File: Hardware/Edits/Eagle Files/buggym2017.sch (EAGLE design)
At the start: 6 parts, among them IC1 4001N, IC2 4075N, IC3 BCC, IC4 L293E

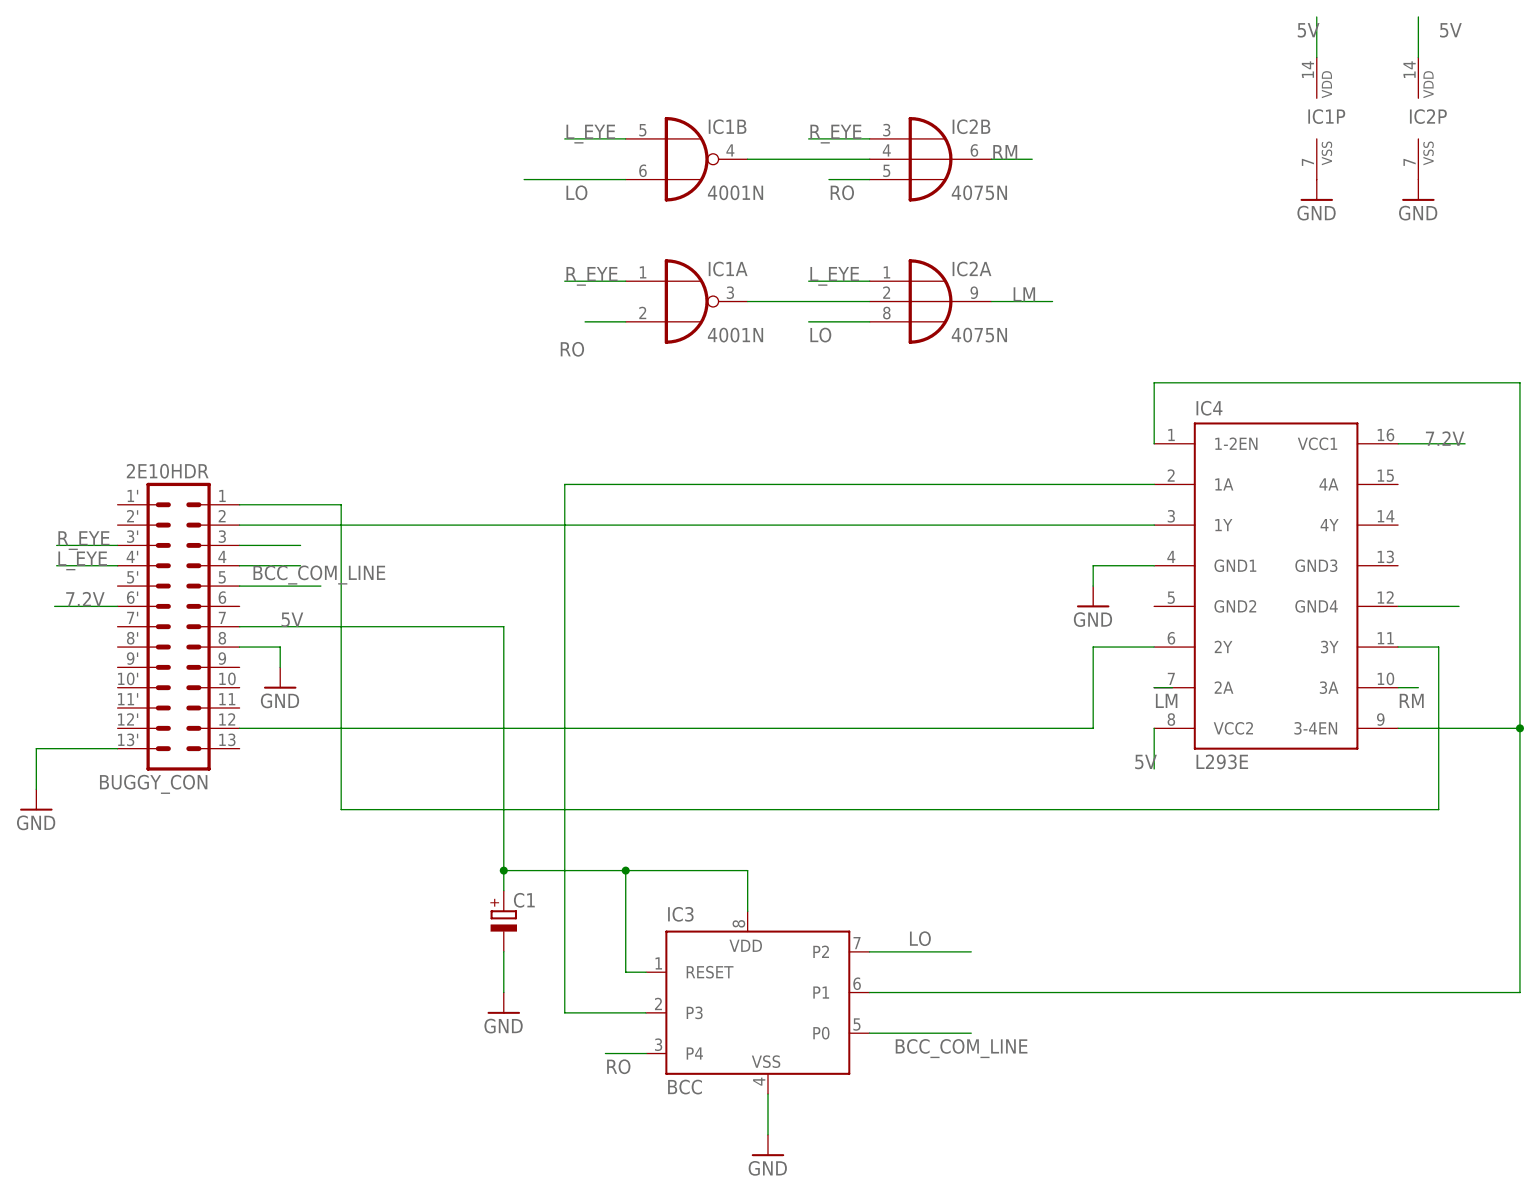
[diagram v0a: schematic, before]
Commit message: Work Done in Week 3  HardwareLab
Work done in Multisim and Eagle
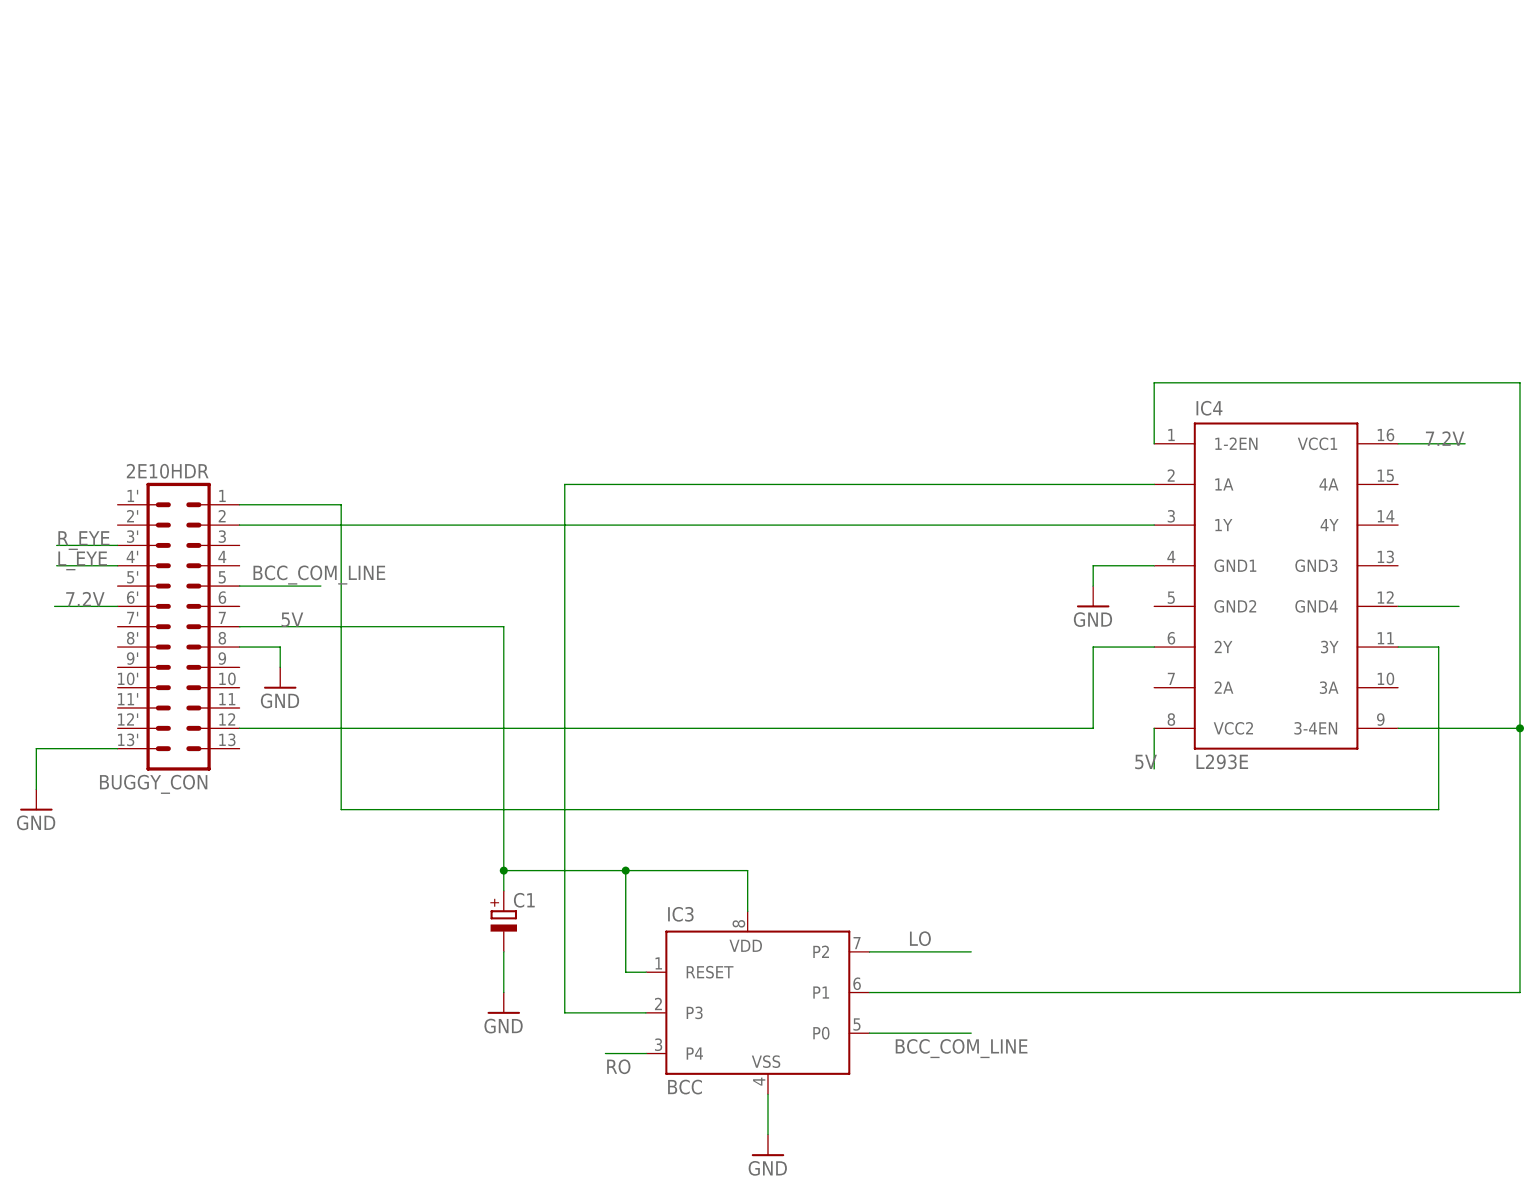
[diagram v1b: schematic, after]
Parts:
- removed IC1: 4001N, 40xx:4001N
- removed IC2: 4075N, 40xx:4075N
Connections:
- removed net LM: IC2A.O
- removed net N$1: IC1A.O, IC2A.I1
- removed net N$4: IC1B.O, IC2B.I1
- removed net RM: IC2B.O
- net GND: no longer IC1P.VSS, IC2P.VSS
- net L_EYE: no longer BUGGY_CON.4
- net R_EYE: no longer BUGGY_CON.3
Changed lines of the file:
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@@
 <?xml version="1.0" encoding="utf-8"?>
 <!DOCTYPE eagle SYSTEM "eagle.dtd">
-<eagle version="7.7.0">
+<eagle version="7.3.0">
 <drawing>
 <settings>
@@
 <part name="GND1" library="supply1" deviceset="GND" device=""/>
 <part name="GND3" library="supply1" deviceset="GND" device=""/>
-<part name="IC1" library="40xx" deviceset="4001" device="N"/>
-<part name="IC2" library="40xx" deviceset="4075" device="N"/>
-<part name="GND4" library="supply1" deviceset="GND" device=""/>
-<part name="GND5" library="supply1" deviceset="GND" device=""/>
 </parts>
 <sheets>
@@
 <instance part="GND1" gate="1" x="-35.56" y="15.24"/>
 <instance part="GND3" gate="1" x="-66.04" y="0"/>
-<instance part="IC1" gate="A" x="15.24" y="63.5"/>
-<instance part="IC2" gate="A" x="45.72" y="63.5"/>
-<instance part="IC2" gate="B" x="45.72" y="81.28"/>
-<instance part="IC1" gate="B" x="15.24" y="81.28"/>
-<instance part="IC1" gate="P" x="93.98" y="86.36"/>
-<instance part="IC2" gate="P" x="106.68" y="86.36"/>
-<instance part="GND4" gate="1" x="93.98" y="76.2"/>
-<instance part="GND5" gate="1" x="106.68" y="76.2"/>
 </instances>
 <busses>
@@
 <wire x1="38.1" y1="-17.78" x2="50.8" y2="-17.78" width="0.1524" layer="91"/>
 <label x="42.926" y="-17.018" size="1.778" layer="95"/>
-</segment>
-<segment>
-<wire x1="30.48" y1="60.96" x2="38.1" y2="60.96" width="0.1524" layer="91"/>
-<label x="30.48" y="58.42" size="1.778" layer="95"/>
-</segment>
-<segment>
-<wire x1="-5.08" y1="78.74" x2="7.62" y2="78.74" width="0.1524" layer="91"/>
-<label x="0" y="76.2" size="1.778" layer="95"/>
 </segment>
 </net>
@@
 <wire x1="-7.62" y1="22.86" x2="-40.64" y2="22.86" width="0.1524" layer="91"/>
 </segment>
-<segment>
-<wire x1="93.98" y1="99.06" x2="93.98" y2="93.98" width="0.1524" layer="91"/>
-<label x="91.44" y="96.52" size="1.778" layer="95"/>
-</segment>
-<segment>
-<wire x1="106.68" y1="93.98" x2="106.68" y2="99.06" width="0.1524" layer="91"/>
-<label x="109.22" y="96.52" size="1.778" layer="95"/>
-</segment>
 </net>
 <net name="GND" class="0">
@@
 <pinref part="BUGGY_CON" gate="G$1" pin="13'"/>
 <wire x1="-66.04" y1="7.62" x2="-55.88" y2="7.62" width="0.1524" layer="91"/>
-</segment>
-<segment>
-<pinref part="IC1" gate="P" pin="VSS"/>
-<pinref part="GND4" gate="1" pin="GND"/>
-</segment>
-<segment>
-<pinref part="IC2" gate="P" pin="VSS"/>
-<pinref part="GND5" gate="1" pin="GND"/>
 </segment>
 </net>
@@
 <label x="5.08" y="-33.02" size="1.778" layer="95"/>
 </segment>
-<segment>
-<wire x1="2.54" y1="60.96" x2="7.62" y2="60.96" width="0.1524" layer="91"/>
-<label x="2.54" y="58.42" size="1.778" layer="95" rot="R180"/>
-</segment>
-<segment>
-<wire x1="33.02" y1="78.74" x2="38.1" y2="78.74" width="0.1524" layer="91"/>
-<label x="33.02" y="76.2" size="1.778" layer="95"/>
-</segment>
 </net>
 <net name="R_EYE" class="0">
@@
 <label x="-63.5" y="33.02" size="1.778" layer="95"/>
 </segment>
-<segment>
-<wire x1="7.62" y1="66.04" x2="0" y2="66.04" width="0.1524" layer="91"/>
-<label x="0" y="66.04" size="1.778" layer="95"/>
-</segment>
-<segment>
-<pinref part="BUGGY_CON" gate="G$1" pin="3"/>
-<wire x1="-33.02" y1="33.02" x2="-40.64" y2="33.02" width="0.1524" layer="91"/>
-</segment>
-<segment>
-<wire x1="38.1" y1="83.82" x2="30.48" y2="83.82" width="0.1524" layer="91"/>
-<label x="30.48" y="83.82" size="1.778" layer="95"/>
-</segment>
 </net>
 <net name="L_EYE" class="0">
@@
 <wire x1="-55.88" y1="30.48" x2="-63.5" y2="30.48" width="0.1524" layer="91"/>
 <label x="-63.5" y="30.48" size="1.778" layer="95"/>
-</segment>
-<segment>
-<wire x1="30.48" y1="66.04" x2="38.1" y2="66.04" width="0.1524" layer="91"/>
-<label x="30.48" y="66.04" size="1.778" layer="95"/>
-</segment>
-<segment>
-<pinref part="BUGGY_CON" gate="G$1" pin="4"/>
-<wire x1="-40.64" y1="30.48" x2="-33.02" y2="30.48" width="0.1524" layer="91"/>
-</segment>
-<segment>
-<wire x1="0" y1="83.82" x2="7.62" y2="83.82" width="0.1524" layer="91"/>
-<label x="0" y="83.82" size="1.778" layer="95"/>
 </segment>
 </net>
@@
 </segment>
 </net>
-<net name="N$1" class="0">
-<segment>
-<pinref part="IC1" gate="A" pin="O"/>
-<pinref part="IC2" gate="A" pin="I1"/>
-<wire x1="22.86" y1="63.5" x2="38.1" y2="63.5" width="0.1524" layer="91"/>
-</segment>
-</net>
-<net name="LM" class="0">
-<segment>
-<pinref part="IC2" gate="A" pin="O"/>
-<wire x1="53.34" y1="63.5" x2="60.96" y2="63.5" width="0.1524" layer="91"/>
-<label x="55.88" y="63.5" size="1.778" layer="95"/>
-</segment>
-<segment>
-<wire x1="75.946" y1="15.24" x2="73.66" y2="15.24" width="0.1524" layer="91"/>
-<label x="73.66" y="12.7" size="1.778" layer="95"/>
-</segment>
-</net>
-<net name="RM" class="0">
-<segment>
-<pinref part="IC2" gate="B" pin="O"/>
-<wire x1="53.34" y1="81.28" x2="58.42" y2="81.28" width="0.1524" layer="91"/>
-<label x="53.34" y="81.28" size="1.778" layer="95"/>
-</segment>
-<segment>
-<wire x1="104.14" y1="15.24" x2="106.68" y2="15.24" width="0.1524" layer="91"/>
-<label x="104.14" y="12.7" size="1.778" layer="95"/>
-</segment>
-</net>
-<net name="N$4" class="0">
-<segment>
-<pinref part="IC1" gate="B" pin="O"/>
-<pinref part="IC2" gate="B" pin="I1"/>
-<wire x1="22.86" y1="81.28" x2="38.1" y2="81.28" width="0.1524" layer="91"/>
-</segment>
-</net>

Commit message: Tidy
Tidied up filesystem from HW Lab Week 3
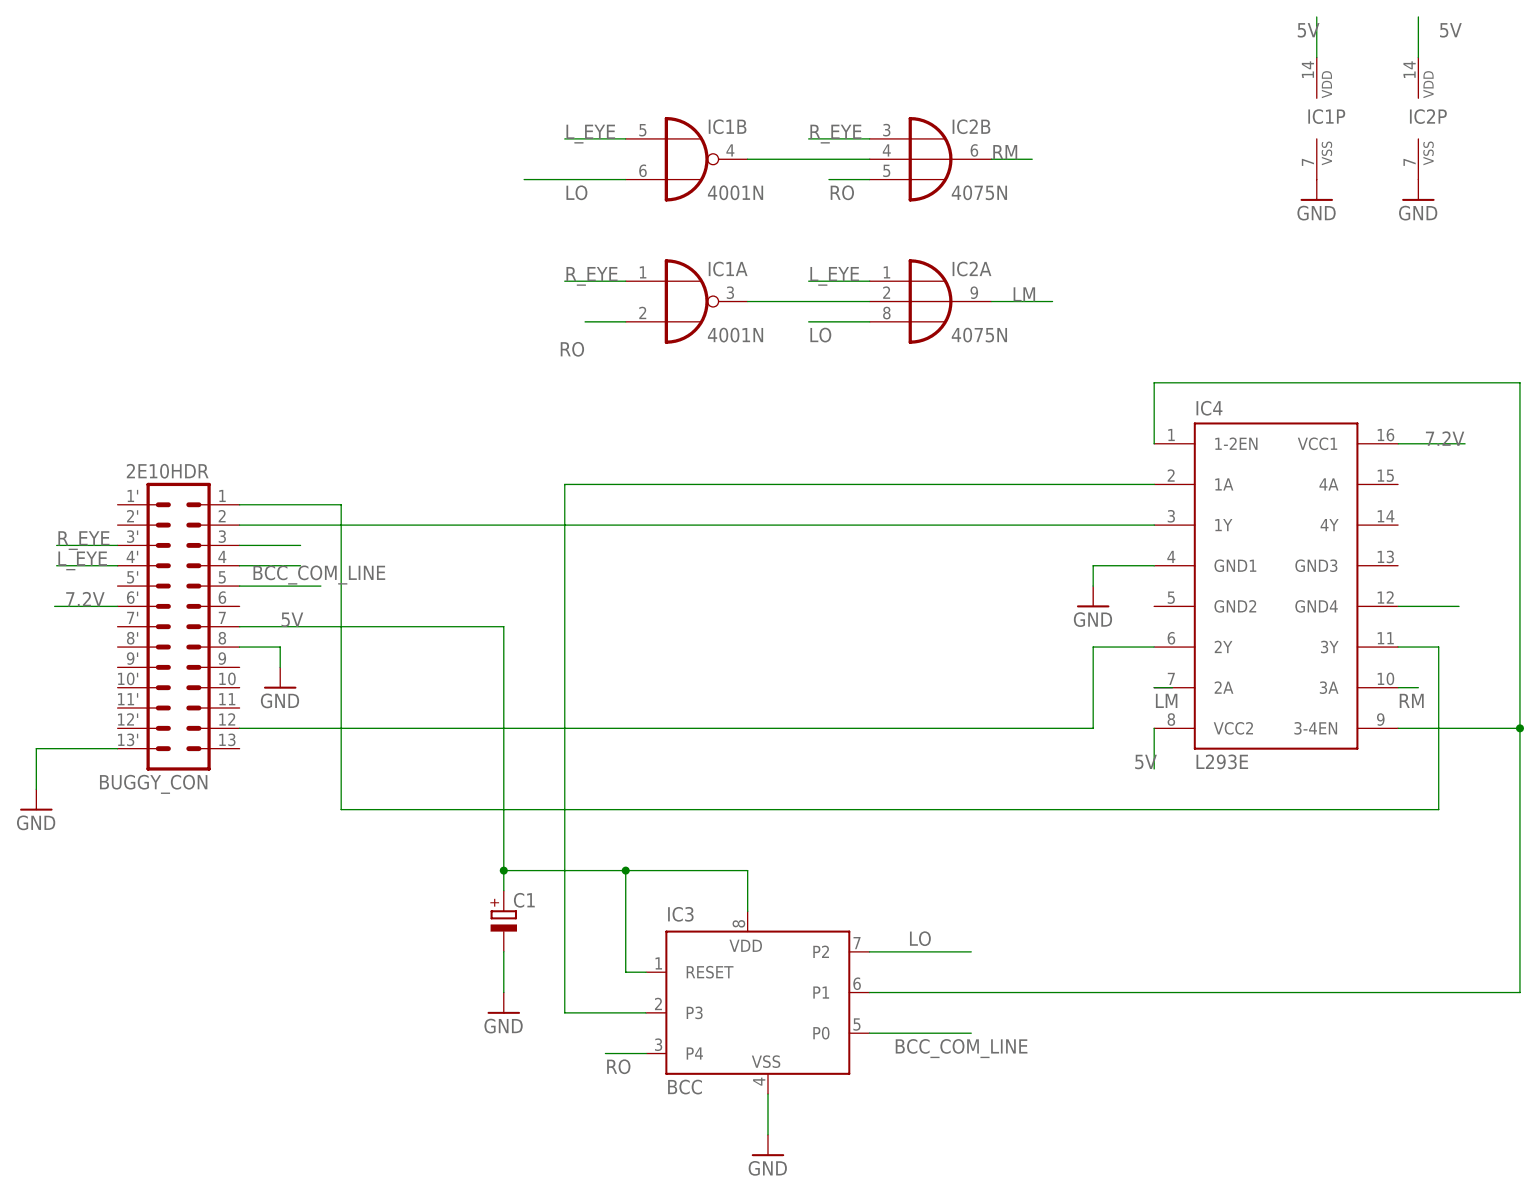
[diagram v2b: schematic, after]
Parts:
- added IC1: 4001N, 40xx:4001N
- added IC2: 4075N, 40xx:4075N
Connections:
- new net LM: IC2A.O
- new net N$1: IC1A.O, IC2A.I1
- new net N$4: IC1B.O, IC2B.I1
- new net RM: IC2B.O
- net GND: now also IC1P.VSS, IC2P.VSS
- net L_EYE: now also BUGGY_CON.4
- net R_EYE: now also BUGGY_CON.3
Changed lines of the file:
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@@
 <?xml version="1.0" encoding="utf-8"?>
 <!DOCTYPE eagle SYSTEM "eagle.dtd">
-<eagle version="7.3.0">
+<eagle version="7.7.0">
 <drawing>
 <settings>
@@
 <part name="GND1" library="supply1" deviceset="GND" device=""/>
 <part name="GND3" library="supply1" deviceset="GND" device=""/>
+<part name="IC1" library="40xx" deviceset="4001" device="N"/>
+<part name="IC2" library="40xx" deviceset="4075" device="N"/>
+<part name="GND4" library="supply1" deviceset="GND" device=""/>
+<part name="GND5" library="supply1" deviceset="GND" device=""/>
 </parts>
 <sheets>
@@
 <instance part="GND1" gate="1" x="-35.56" y="15.24"/>
 <instance part="GND3" gate="1" x="-66.04" y="0"/>
+<instance part="IC1" gate="A" x="15.24" y="63.5"/>
+<instance part="IC2" gate="A" x="45.72" y="63.5"/>
+<instance part="IC2" gate="B" x="45.72" y="81.28"/>
+<instance part="IC1" gate="B" x="15.24" y="81.28"/>
+<instance part="IC1" gate="P" x="93.98" y="86.36"/>
+<instance part="IC2" gate="P" x="106.68" y="86.36"/>
+<instance part="GND4" gate="1" x="93.98" y="76.2"/>
+<instance part="GND5" gate="1" x="106.68" y="76.2"/>
 </instances>
 <busses>
@@
 <wire x1="38.1" y1="-17.78" x2="50.8" y2="-17.78" width="0.1524" layer="91"/>
 <label x="42.926" y="-17.018" size="1.778" layer="95"/>
+</segment>
+<segment>
+<wire x1="30.48" y1="60.96" x2="38.1" y2="60.96" width="0.1524" layer="91"/>
+<label x="30.48" y="58.42" size="1.778" layer="95"/>
+</segment>
+<segment>
+<wire x1="-5.08" y1="78.74" x2="7.62" y2="78.74" width="0.1524" layer="91"/>
+<label x="0" y="76.2" size="1.778" layer="95"/>
 </segment>
 </net>
@@
 <wire x1="-7.62" y1="22.86" x2="-40.64" y2="22.86" width="0.1524" layer="91"/>
 </segment>
+<segment>
+<wire x1="93.98" y1="99.06" x2="93.98" y2="93.98" width="0.1524" layer="91"/>
+<label x="91.44" y="96.52" size="1.778" layer="95"/>
+</segment>
+<segment>
+<wire x1="106.68" y1="93.98" x2="106.68" y2="99.06" width="0.1524" layer="91"/>
+<label x="109.22" y="96.52" size="1.778" layer="95"/>
+</segment>
 </net>
 <net name="GND" class="0">
@@
 <pinref part="BUGGY_CON" gate="G$1" pin="13'"/>
 <wire x1="-66.04" y1="7.62" x2="-55.88" y2="7.62" width="0.1524" layer="91"/>
+</segment>
+<segment>
+<pinref part="IC1" gate="P" pin="VSS"/>
+<pinref part="GND4" gate="1" pin="GND"/>
+</segment>
+<segment>
+<pinref part="IC2" gate="P" pin="VSS"/>
+<pinref part="GND5" gate="1" pin="GND"/>
 </segment>
 </net>
@@
 <label x="5.08" y="-33.02" size="1.778" layer="95"/>
 </segment>
+<segment>
+<wire x1="2.54" y1="60.96" x2="7.62" y2="60.96" width="0.1524" layer="91"/>
+<label x="2.54" y="58.42" size="1.778" layer="95" rot="R180"/>
+</segment>
+<segment>
+<wire x1="33.02" y1="78.74" x2="38.1" y2="78.74" width="0.1524" layer="91"/>
+<label x="33.02" y="76.2" size="1.778" layer="95"/>
+</segment>
 </net>
 <net name="R_EYE" class="0">
@@
 <label x="-63.5" y="33.02" size="1.778" layer="95"/>
 </segment>
+<segment>
+<wire x1="7.62" y1="66.04" x2="0" y2="66.04" width="0.1524" layer="91"/>
+<label x="0" y="66.04" size="1.778" layer="95"/>
+</segment>
+<segment>
+<pinref part="BUGGY_CON" gate="G$1" pin="3"/>
+<wire x1="-33.02" y1="33.02" x2="-40.64" y2="33.02" width="0.1524" layer="91"/>
+</segment>
+<segment>
+<wire x1="38.1" y1="83.82" x2="30.48" y2="83.82" width="0.1524" layer="91"/>
+<label x="30.48" y="83.82" size="1.778" layer="95"/>
+</segment>
 </net>
 <net name="L_EYE" class="0">
@@
 <wire x1="-55.88" y1="30.48" x2="-63.5" y2="30.48" width="0.1524" layer="91"/>
 <label x="-63.5" y="30.48" size="1.778" layer="95"/>
+</segment>
+<segment>
+<wire x1="30.48" y1="66.04" x2="38.1" y2="66.04" width="0.1524" layer="91"/>
+<label x="30.48" y="66.04" size="1.778" layer="95"/>
+</segment>
+<segment>
+<pinref part="BUGGY_CON" gate="G$1" pin="4"/>
+<wire x1="-40.64" y1="30.48" x2="-33.02" y2="30.48" width="0.1524" layer="91"/>
+</segment>
+<segment>
+<wire x1="0" y1="83.82" x2="7.62" y2="83.82" width="0.1524" layer="91"/>
+<label x="0" y="83.82" size="1.778" layer="95"/>
 </segment>
 </net>
@@
 </segment>
 </net>
+<net name="N$1" class="0">
+<segment>
+<pinref part="IC1" gate="A" pin="O"/>
+<pinref part="IC2" gate="A" pin="I1"/>
+<wire x1="22.86" y1="63.5" x2="38.1" y2="63.5" width="0.1524" layer="91"/>
+</segment>
+</net>
+<net name="LM" class="0">
+<segment>
+<pinref part="IC2" gate="A" pin="O"/>
+<wire x1="53.34" y1="63.5" x2="60.96" y2="63.5" width="0.1524" layer="91"/>
+<label x="55.88" y="63.5" size="1.778" layer="95"/>
+</segment>
+<segment>
+<wire x1="75.946" y1="15.24" x2="73.66" y2="15.24" width="0.1524" layer="91"/>
+<label x="73.66" y="12.7" size="1.778" layer="95"/>
+</segment>
+</net>
+<net name="RM" class="0">
+<segment>
+<pinref part="IC2" gate="B" pin="O"/>
+<wire x1="53.34" y1="81.28" x2="58.42" y2="81.28" width="0.1524" layer="91"/>
+<label x="53.34" y="81.28" size="1.778" layer="95"/>
+</segment>
+<segment>
+<wire x1="104.14" y1="15.24" x2="106.68" y2="15.24" width="0.1524" layer="91"/>
+<label x="104.14" y="12.7" size="1.778" layer="95"/>
+</segment>
+</net>
+<net name="N$4" class="0">
+<segment>
+<pinref part="IC1" gate="B" pin="O"/>
+<pinref part="IC2" gate="B" pin="I1"/>
+<wire x1="22.86" y1="81.28" x2="38.1" y2="81.28" width="0.1524" layer="91"/>
+</segment>
+</net>
